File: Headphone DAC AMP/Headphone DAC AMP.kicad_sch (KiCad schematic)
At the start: 3 parts

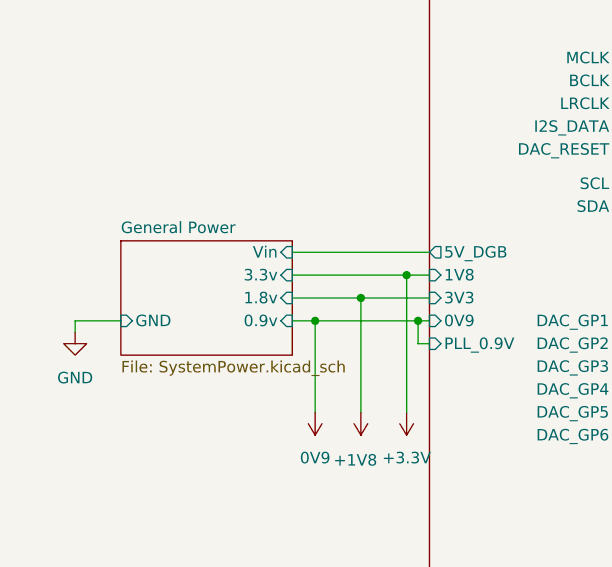
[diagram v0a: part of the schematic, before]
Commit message: Routing Complete!
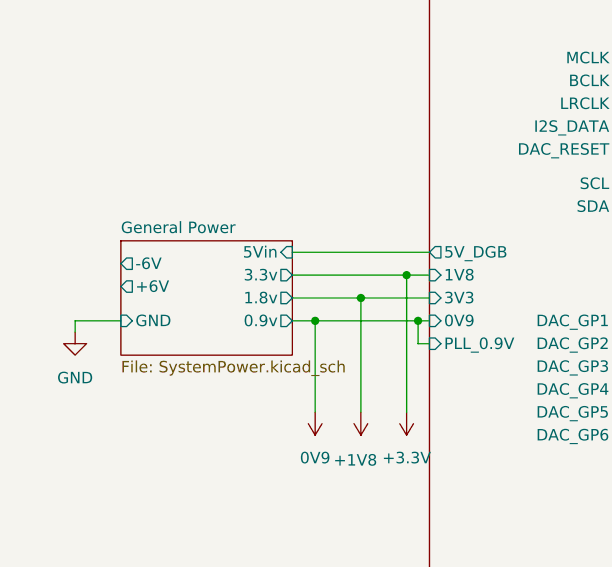
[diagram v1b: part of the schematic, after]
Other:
- sheet General Power ports: added +6V, -6V, 5Vin; removed Vin
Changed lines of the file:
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@@
 			)
 		)
-		(pin "0.9v" input
+		(pin "0.9v" output
 			(at 53.34 100.33 0)
 			(effects
@@
 			)
 		)
-		(pin "1.8v" input
+		(pin "1.8v" output
 			(at 53.34 97.79 0)
 			(effects
@@
 			)
 		)
-		(pin "3.3v" input
+		(pin "3.3v" output
 			(at 53.34 95.25 0)
-			(effects
-				(font
-					(size 1.27 1.27)
-				)
-				(justify right)
-			)
-		)
-		(pin "Vin" input
-			(at 53.34 92.71 0)
 			(effects
 				(font
@@
 			)
 		)
+		(pin "+6V" output
+			(at 34.29 96.52 180)
+			(effects
+				(font
+					(size 1.27 1.27)
+				)
+				(justify left)
+			)
+		)
+		(pin "-6V" output
+			(at 34.29 93.98 180)
+			(effects
+				(font
+					(size 1.27 1.27)
+				)
+				(justify left)
+			)
+		)
+		(pin "5Vin" input
+			(at 53.34 92.71 0)
+			(effects
+				(font
+					(size 1.27 1.27)
+				)
+				(justify right)
+			)
+		)
